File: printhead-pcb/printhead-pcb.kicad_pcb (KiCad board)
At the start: 2 copper layers, 35 x 35 mm, 4 parts, among them U3 EMC2302-2-AIZL-TR, U4 EMC2302-2-AIZL-TR, U5 ADS1015IDGS, U6 PCA9536D

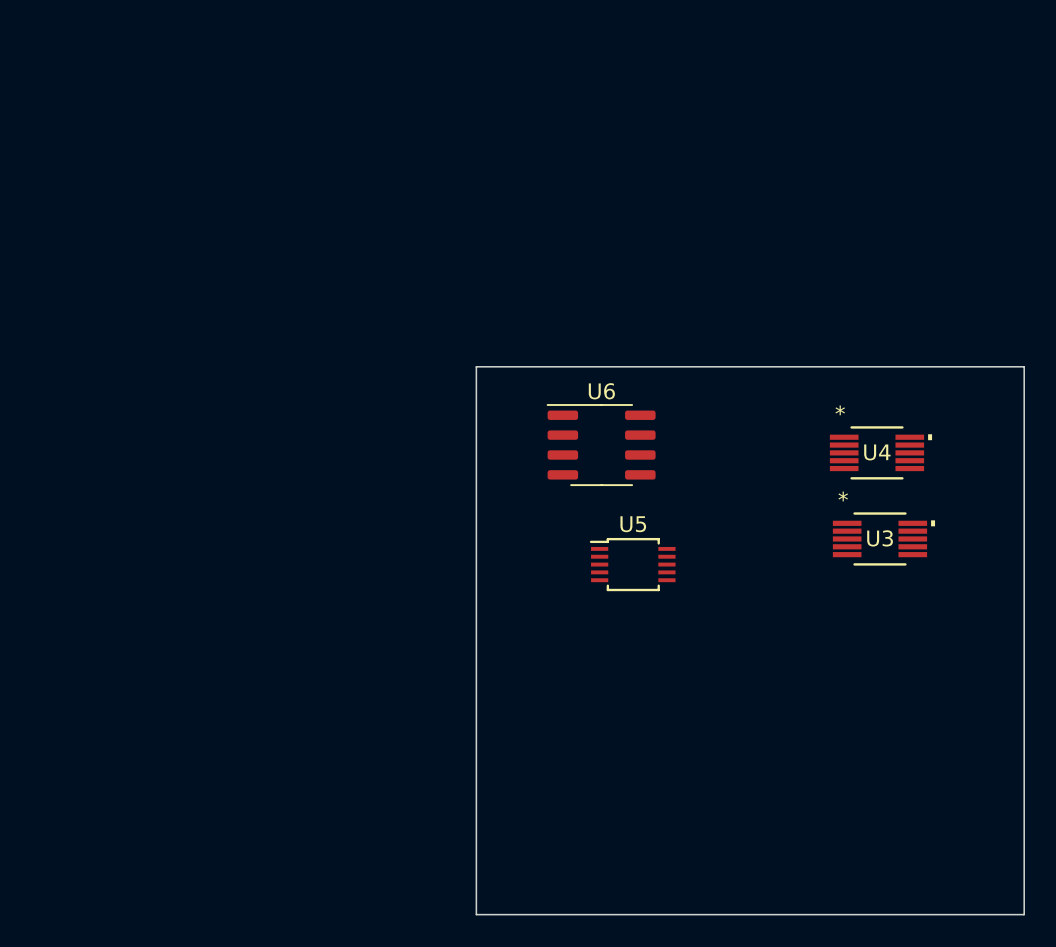
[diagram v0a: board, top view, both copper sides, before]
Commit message: circuit finished?
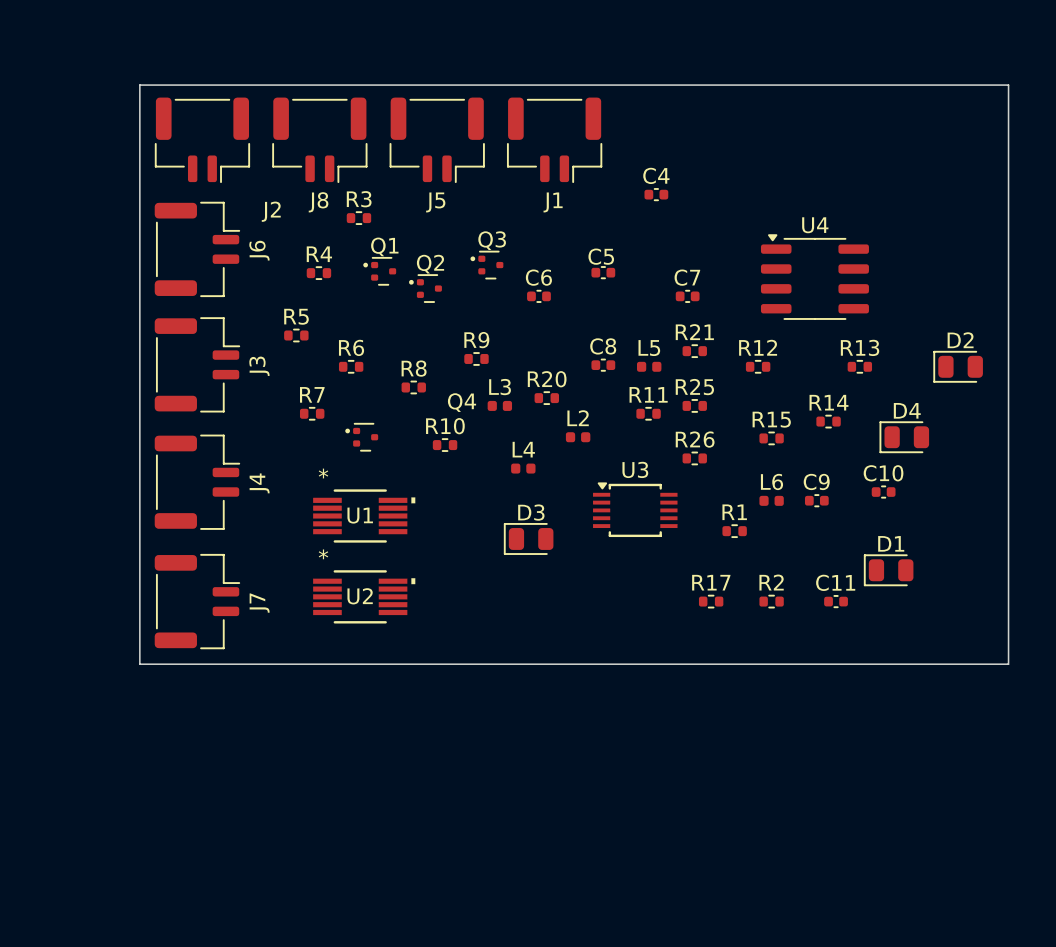
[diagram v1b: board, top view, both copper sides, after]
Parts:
- removed U5: ADS1015IDGS, Package_SO:TSSOP-10_3x3mm_P0.5mm
- removed U6: PCA9536D, Package_SO:SOIC-8_3.9x4.9mm_P1.27mm
- added C10: 0.22µF, Capacitor_SMD:C_0402_1005Metric, F.Cu at (154.0, 74.5)
- added C11: 0.1µF, Capacitor_SMD:C_0402_1005Metric, F.Cu at (151.0, 81.5)
- added C4: 0.1µF, Capacitor_SMD:C_0402_1005Metric, F.Cu at (139.5, 55.5)
- added C5: 0.1µF, Capacitor_SMD:C_0402_1005Metric, F.Cu at (136.1, 60.5)
- added C6: 0.1µF, Capacitor_SMD:C_0402_1005Metric, F.Cu at (132.0, 62.0)
- added C7: 0.1µFC, Capacitor_SMD:C_0402_1005Metric, F.Cu at (141.5, 62.0)
- added C8: 0.1µF, Capacitor_SMD:C_0402_1005Metric, F.Cu at (136.1, 66.4)
- added C9: 1µF, Capacitor_SMD:C_0402_1005Metric, F.Cu at (149.8, 75.1)
- added D1: GREEN, LED_SMD:LED_0805_2012Metric, F.Cu at (154.5, 79.5)
- added D2: YELLOW, LED_SMD:LED_0805_2012Metric, F.Cu at (158.9, 66.5)
- added D3: BLUE, LED_SMD:LED_0805_2012Metric, F.Cu at (131.5, 77.5)
- added D4: YELLOW, LED_SMD:LED_0805_2012Metric, F.Cu at (155.5, 71.0)
- added J1: FAN0, Connector_JST:JST_GH_SM02B-GHS-TB_1x02-1MP_P1.25mm_Horizontal, F.Cu at (133.0, 52.0)
- added J2: FAN2, Connector_JST:JST_GH_SM02B-GHS-TB_1x02-1MP_P1.25mm_Horizontal, F.Cu at (110.5, 52.0)
- added J3: FAN1, Connector_JST:JST_GH_SM02B-GHS-TB_1x02-1MP_P1.25mm_Horizontal, F.Cu at (110.2, 66.4)
- added J4: FAN3, Connector_JST:JST_GH_SM02B-GHS-TB_1x02-1MP_P1.25mm_Horizontal, F.Cu at (110.2, 73.9)
- added J5: T0, Connector_JST:JST_GH_SM02B-GHS-TB_1x02-1MP_P1.25mm_Horizontal, F.Cu at (125.5, 52.0)
- added J6: T1, Connector_JST:JST_GH_SM02B-GHS-TB_1x02-1MP_P1.25mm_Horizontal, F.Cu at (110.2, 59.0)
- added J7: T2, Connector_JST:JST_GH_SM02B-GHS-TB_1x02-1MP_P1.25mm_Horizontal, F.Cu at (110.2, 81.5)
- added J8: T3, Connector_JST:JST_GH_SM02B-GHS-TB_1x02-1MP_P1.25mm_Horizontal, F.Cu at (118.0, 52.0)
- added L2: L, Inductor_SMD:L_0402_1005Metric, F.Cu at (134.5, 71.0)
- added L3: L, Inductor_SMD:L_0402_1005Metric, F.Cu at (129.5, 69.0)
- added L4: L, Inductor_SMD:L_0402_1005Metric, F.Cu at (131.0, 73.0)
- added L5: L, Inductor_SMD:L_0402_1005Metric, F.Cu at (139.0, 66.5)
- added L6: L, Inductor_SMD:L_0402_1005Metric, F.Cu at (146.9, 75.1)
- added Q1: DTC143E, Package_TO_SOT_SMD:SOT-723, F.Cu at (122.1, 60.4)
- added Q2: DTC143E, Package_TO_SOT_SMD:SOT-723, F.Cu at (125.0, 61.5)
- added Q3: DTC143E, Package_TO_SOT_SMD:SOT-723, F.Cu at (128.9, 60.0)
- added Q4: DTC143E, Package_TO_SOT_SMD:SOT-723, F.Cu at (120.9, 71.0)
- added R1: 10k, Resistor_SMD:R_0402_1005Metric, F.Cu at (144.5, 77.0)
- added R10: 10k, Resistor_SMD:R_0402_1005Metric, F.Cu at (126.0, 71.5)
- added R11: 330, Resistor_SMD:R_0402_1005Metric, F.Cu at (139.0, 69.5)
- added R12: 330, Resistor_SMD:R_0402_1005Metric, F.Cu at (146.0, 66.5)
- added R13: 330, Resistor_SMD:R_0402_1005Metric, F.Cu at (152.5, 66.5)
- added R14: 10k, Resistor_SMD:R_0402_1005Metric, F.Cu at (150.5, 70.0)
- added R15: 10k, Resistor_SMD:R_0402_1005Metric, F.Cu at (146.9, 71.1)
- added R17: 1k, Resistor_SMD:R_0402_1005Metric, F.Cu at (143.0, 81.5)
- added R2: 10k, Resistor_SMD:R_0402_1005Metric, F.Cu at (146.9, 81.5)
- added R20: 1k8, Resistor_SMD:R_0402_1005Metric, F.Cu at (132.5, 68.5)
- added R21: 1k8, Resistor_SMD:R_0402_1005Metric, F.Cu at (142.0, 65.5)
- added R25: 1k8, Resistor_SMD:R_0402_1005Metric, F.Cu at (142.0, 69.0)
- added R26: 1k8, Resistor_SMD:R_0402_1005Metric, F.Cu at (142.0, 72.4)
- added R3: 10k, Resistor_SMD:R_0402_1005Metric, F.Cu at (120.5, 57.0)
- added R4: 10k, Resistor_SMD:R_0402_1005Metric, F.Cu at (117.9, 60.5)
- added R5: 3k3, Resistor_SMD:R_0402_1005Metric, F.Cu at (116.5, 64.5)
- added R6: 3k3, Resistor_SMD:R_0402_1005Metric, F.Cu at (120.0, 66.5)
- added R7: 10k, Resistor_SMD:R_0402_1005Metric, F.Cu at (117.5, 69.5)
- added R8: 10k, Resistor_SMD:R_0402_1005Metric, F.Cu at (124.0, 67.8)
- added R9: 10k, Resistor_SMD:R_0402_1005Metric, F.Cu at (128.0, 66.0)
- added U1: EMC2302-1-AIZL-TR, EMC2302-1-AIZL-TR:MSOP10_MC_MCH-M, F.Cu at (120.6, 76.0)
- added U2: EMC2302-2-AIZL-TR, EMC2302-1-AIZL-TR:MSOP10_MC_MCH-M, F.Cu at (120.6, 81.2)
- U3: value EMC2302-2-AIZL-TR -> ADS1015IDGS; footprint EMC2302-2-AIZL-TR:MSOP10_MC_MCH-M -> Package_SO:TSSOP-10_3x3mm_P0.5mm
- U4: value EMC2302-2-AIZL-TR -> PCA9536D; footprint EMC2302-2-AIZL-TR:MSOP10_MC_MCH-M -> Package_SO:SOIC-8_3.9x4.9mm_P1.27mm
- moved U3 15.7 mm to (138.2, 75.7)
- moved U4 11.8 mm to (149.6, 60.9)
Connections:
- U3 pad 1: unconnected-(U3-SMDATA-Pad1) -> GND
- U3 pad 10: unconnected-(U3-*ALERT-Pad10) -> SCL
- U3 pad 2: unconnected-(U3-SMCLK-Pad2) -> Net-(D3-A)
- U3 pad 3: unconnected-(U3-VDD-Pad3) -> GND
- U3 pad 4: unconnected-(U3-GND-Pad4) -> ADC0
- U3 pad 5: unconnected-(U3-PWM1-Pad5) -> ADC1
- U3 pad 6: unconnected-(U3-TACH1-Pad6) -> ADC2
- U3 pad 7: unconnected-(U3-PWM2-Pad7) -> ADC3
- U3 pad 8: unconnected-(U3-TACH2-Pad8) -> +3.3V
- U3 pad 9: unconnected-(U3-CLK-Pad9) -> SDA
- U4 pad 1: unconnected-(U4-SMDATA-Pad1) -> IO0
- U4 pad 2: unconnected-(U4-SMCLK-Pad2) -> IO1
- U4 pad 3: unconnected-(U4-VDD-Pad3) -> IO2
- U4 pad 4: unconnected-(U4-GND-Pad4) -> GND
- U4 pad 5: unconnected-(U4-PWM1-Pad5) -> IO3
- U4 pad 6: unconnected-(U4-TACH1-Pad6) -> SDA
- U4 pad 7: unconnected-(U4-PWM2-Pad7) -> SDA
- U4 pad 8: unconnected-(U4-TACH2-Pad8) -> +3.3V
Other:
- board size 35 x 35 mm -> 55.5 x 37 mm
- board text added: "*"

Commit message: layout
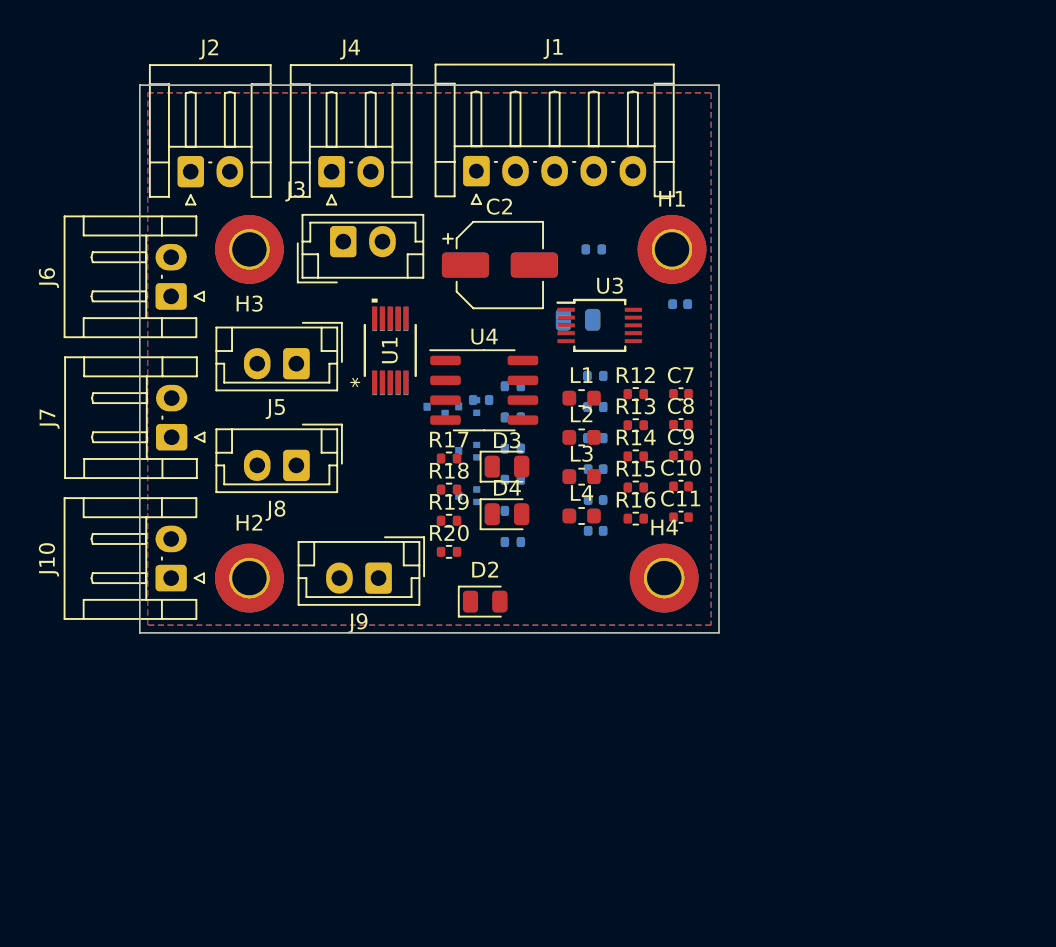
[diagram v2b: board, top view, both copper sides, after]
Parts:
- removed L5, L6: L, Inductor_SMD:L_0402_1005Metric
- removed R21, R25, R26: 1k8, Resistor_SMD:R_0402_1005Metric
- added C1: 0.1µF, Capacitor_SMD:CP_Elec_5x3, B.Cu at (129.5, 60.0)
- added C2: 0.1µF, Capacitor_SMD:CP_Elec_5x3, F.Cu at (129.5, 60.0)
- added C3: 0.22µF, Capacitor_SMD:C_0402_1005Metric, B.Cu at (135.6, 75.0)
- added H1: MountingHole_Pad, MountingHole:MountingHole_2.2mm_M2_Pad_TopBottom, F.Cu at (140.5, 59.0)
- added H2: MountingHole_Pad, MountingHole:MountingHole_2.2mm_M2_Pad_TopBottom, F.Cu at (113.5, 80.0)
- added H3: MountingHole_Pad, MountingHole:MountingHole_2.2mm_M2_Pad_TopBottom, F.Cu at (113.5, 59.0)
- added H4: MountingHole_Pad, MountingHole:MountingHole_2.2mm_M2_Pad_TopBottom, F.Cu at (140.0, 80.0)
- added J1: PWR, Connector_JST:JST_EH_S5B-EH_1x05_P2.50mm_Horizontal, F.Cu at (128.0, 54.0)
- added J10: BL_TOUCH, Connector_JST:JST_EH_S2B-EH_1x02_P2.50mm_Horizontal, F.Cu at (108.5, 80.0)
- added L1: L, Inductor_SMD:L_0603_1608Metric, F.Cu at (134.7, 68.5)
- added R16: 4k7, Resistor_SMD:R_0402_1005Metric, F.Cu at (138.2, 76.2)
- added R18: 10k, Resistor_SMD:R_0402_1005Metric, F.Cu at (126.3, 74.3)
- added R19: 330, Resistor_SMD:R_0402_1005Metric, F.Cu at (126.3, 76.3)
- C10: value 0.22µF -> 0.1µFC
- C4: value 0.1µF -> 0.22µF; moved to B.Cu
- C5, C6, D1, Q1, Q2, Q3, Q4, R10, R2, R3, R4, R7, R8, R9: moved to B.Cu
- C7: value 0.1µFC -> 0.1µF
- C9: value 1µF -> 0.1µF
- D2: value YELLOW -> BLUE
- D3: value BLUE -> YELLOW
- J2: renamed from J1; footprint Connector_JST:JST_GH_SM02B-GHS-TB_1x02-1MP_P1.25mm_Horizontal -> Connector_JST:JST_EH_S2B-EH_1x02_P2.50mm_Horizontal
- J3: renamed from J2; footprint Connector_JST:JST_GH_SM02B-GHS-TB_1x02-1MP_P1.25mm_Horizontal -> Connector_JST:JST_EH_B2B-EH-A_1x02_P2.50mm_Vertical
- J4: renamed from J3; footprint Connector_JST:JST_GH_SM02B-GHS-TB_1x02-1MP_P1.25mm_Horizontal -> Connector_JST:JST_EH_S2B-EH_1x02_P2.50mm_Horizontal
- J5: renamed from J4; footprint Connector_JST:JST_GH_SM02B-GHS-TB_1x02-1MP_P1.25mm_Horizontal -> Connector_JST:JST_EH_B2B-EH-A_1x02_P2.50mm_Vertical
- J6: renamed from J5; footprint Connector_JST:JST_GH_SM02B-GHS-TB_1x02-1MP_P1.25mm_Horizontal -> Connector_JST:JST_EH_S2B-EH_1x02_P2.50mm_Horizontal
- J7: renamed from J6; footprint Connector_JST:JST_GH_SM02B-GHS-TB_1x02-1MP_P1.25mm_Horizontal -> Connector_JST:JST_EH_S2B-EH_1x02_P2.50mm_Horizontal
- J8: renamed from J7; footprint Connector_JST:JST_GH_SM02B-GHS-TB_1x02-1MP_P1.25mm_Horizontal -> Connector_JST:JST_EH_B2B-EH-A_1x02_P2.50mm_Vertical
- J9: renamed from J8; footprint Connector_JST:JST_GH_SM02B-GHS-TB_1x02-1MP_P1.25mm_Horizontal -> Connector_JST:JST_EH_B2B-EH-A_1x02_P2.50mm_Vertical
- L2, L3, L4: footprint Inductor_SMD:L_0402_1005Metric -> Inductor_SMD:L_0603_1608Metric
- R1: value 10k -> 1k; moved to B.Cu
- R11: value 330 -> 10k; moved to B.Cu
- R12, R13: value 330 -> 4k7
- R14: value 10k -> 330
- R15: value 10k -> 4k7
- R17: value 1k -> 10k
- R20: value 1k8 -> 330
- R5, R6: value 3k3 -> 10k; moved to B.Cu
- U1: value EMC2302-1-AIZL-TR -> EMC2302-2-AIZL-TR; footprint EMC2302-1-AIZL-TR:MSOP10_MC_MCH-M -> EMC2302-2-AIZL-TR:MSOP10_MC_MCH
- U2: footprint EMC2302-1-AIZL-TR:MSOP10_MC_MCH-M -> EMC2302-2-AIZL-TR:MSOP10_MC_MCH; moved to B.Cu
- moved D2 33.9 mm to (128.6, 81.5)
- moved J9 28.2 mm to (121.8, 80.0)
- moved D4 26.0 mm to (130.0, 75.9)
- moved D1 25.6 mm to (134.5, 63.5), turned to 180 degrees
- moved J2 23.3 mm to (109.8, 54.0), turned to 0 degrees
- moved U4 22.3 mm to (128.5, 68.0)
- moved R3 20.6 mm to (135.6, 71.1), turned to 180 degrees
- moved J6 19.7 mm to (108.5, 62.0), turned to 90 degrees
- moved R17 19.1 mm to (126.3, 72.4)
- moved C4 18.0 mm to (135.6, 73.0), turned to 180 degrees
- moved R2 16.8 mm to (135.6, 69.1), turned to 180 degrees
- moved U2 15.8 mm to (122.5, 65.5), turned to -90 degrees
- moved C6 15.4 mm to (135.6, 77.0), turned to 180 degrees
- moved J4 15.0 mm to (118.8, 54.0), turned to 0 degrees
- moved R13 14.8 mm to (138.2, 70.2)
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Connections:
- C10 pad 1: Net-(C10-Pad1) -> ADC2
- C11 pad 1: Net-(C10-Pad1) -> ADC3
- C4 pad 1: ADC0 -> +3V3
- C5 pad 1: +3.3V -> +12V
- C6 pad 1: ADC0 -> +3V3
- C8 pad 1: ADC0 -> +3.3V
- C9 pad 1: Net-(C10-Pad1) -> ADC1
- D2 pad 2: IO0 -> Net-(D2-A)
- D3 pad 2: Net-(D3-A) -> IO0
- L2 pad 1: TC0 -> TC1
- L2 pad 2: ADC0 -> ADC1
- L3 pad 1: TC0 -> TC2
- L3 pad 2: ADC0 -> ADC2
- L4 pad 1: TC0 -> TC3
- L4 pad 2: ADC0 -> ADC3
- R1 pad 1: +3V3 -> Net-(D1-K)
- R1 pad 2: SDA -> GND
- R10 pad 1: Net-(U2-CLK) -> Net-(U1-CLK)
- R11 pad 1: GND -> Net-(U2-CLK)
- R11 pad 2: Net-(D3-K) -> GND
- R12 pad 1: Net-(D2-K) -> AREF
- R12 pad 2: GND -> ADC0
- R13 pad 1: Net-(D4-K) -> AREF
- R13 pad 2: GND -> ADC1
- R14 pad 1: IO2 -> GND
- R14 pad 2: GND -> Net-(D2-K)
- R15 pad 1: IO3 -> AREF
- R15 pad 2: GND -> ADC2
- R17 pad 1: Net-(D1-K) -> IO3
- R2 pad 2: SCL -> SDA
- R20 pad 1: AREF -> Net-(D4-K)
- R20 pad 2: ADC0 -> GND
- R3 pad 1: Net-(U1-TACH1) -> +3V3
- R3 pad 2: GND -> SCL
- R4 pad 1: Net-(U2-TACH1) -> Net-(U1-TACH1)
- R5 pad 1: Net-(U1-*ALERT) -> Net-(U2-TACH1)
- R6 pad 1: Net-(U2-*ALERT) -> Net-(U1-*ALERT)
- R7 pad 1: Net-(U1-TACH2) -> Net-(U2-*ALERT)
- R8 pad 1: Net-(U2-TACH2) -> Net-(U1-TACH2)
- R9 pad 1: Net-(U1-CLK) -> Net-(U2-TACH2)
- U3 pad 2: Net-(D3-A) -> Net-(D2-A)
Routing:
- added copper zone on B.Cu, net GND
- added copper zone on F.Cu, net GND
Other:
- board size 55.5 x 37 mm -> 37 x 35 mm
- board text removed: "*"

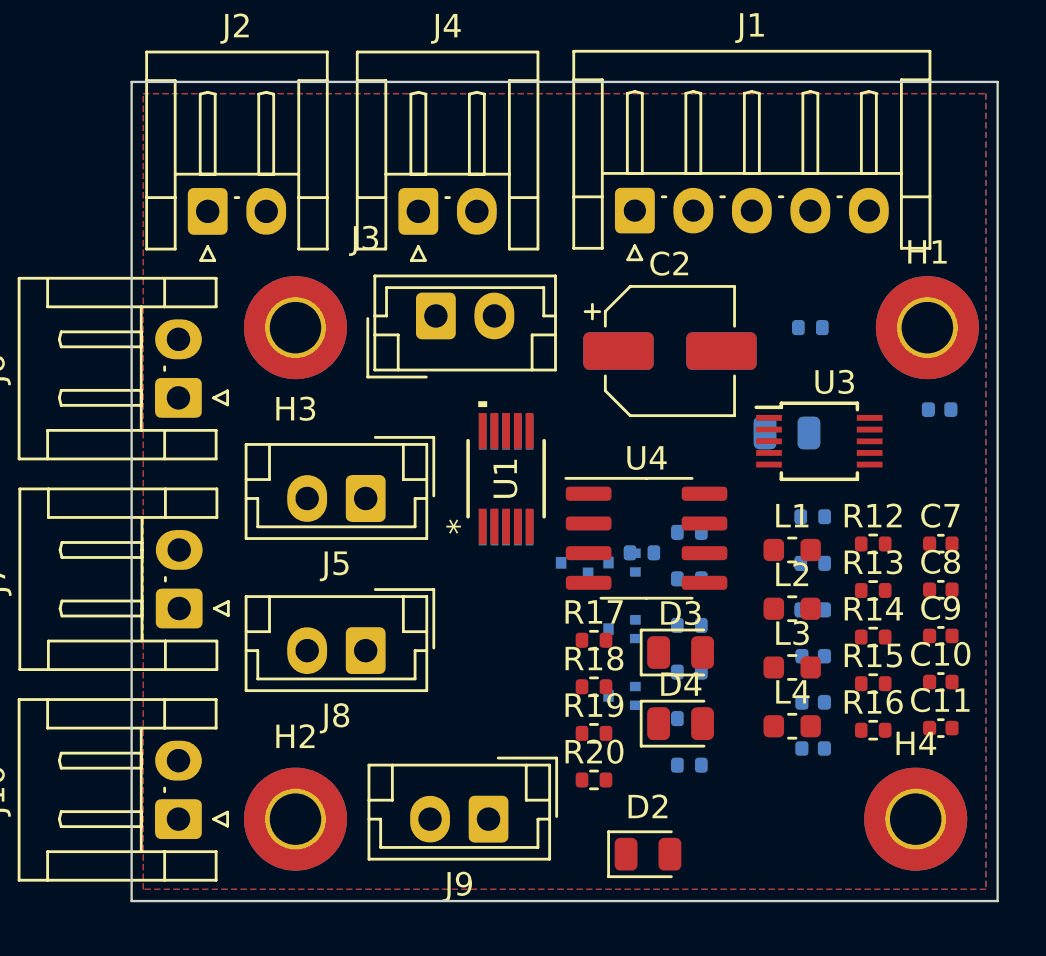
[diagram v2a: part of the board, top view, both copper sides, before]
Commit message: first pcb layout
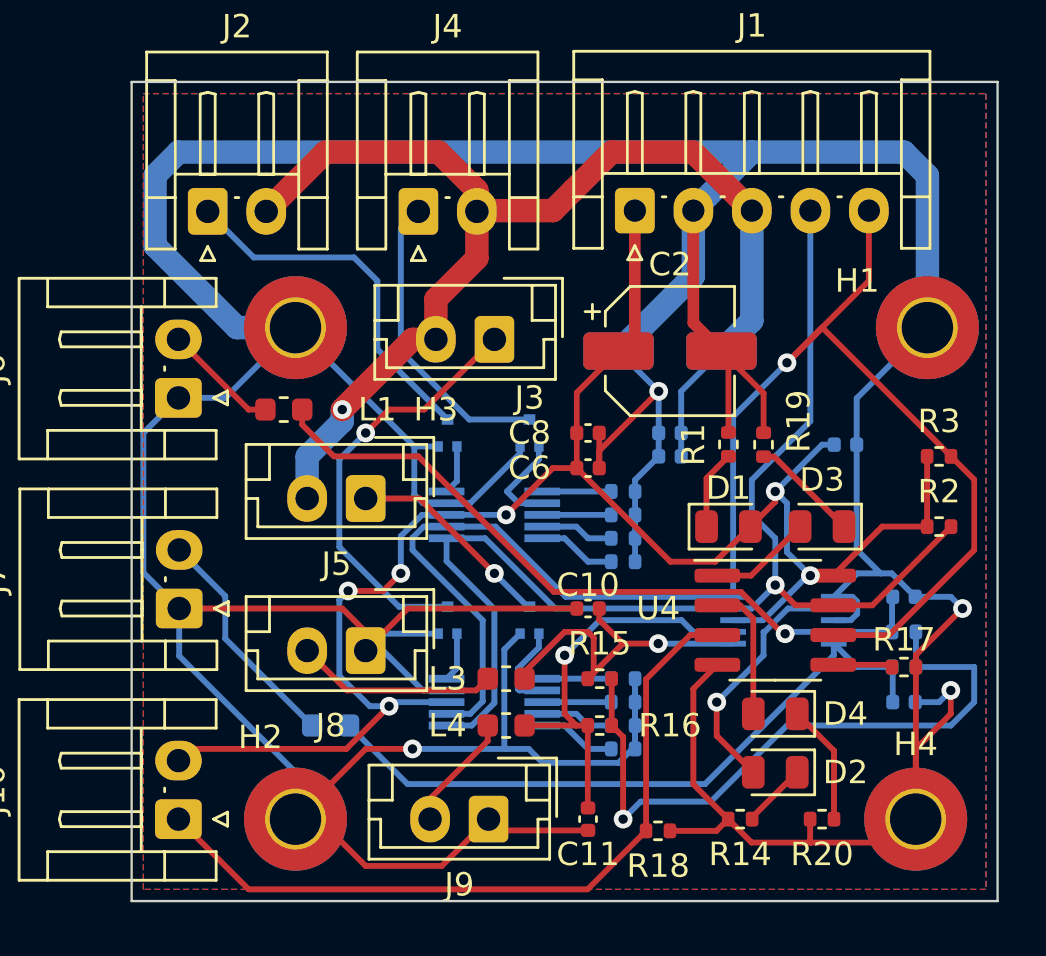
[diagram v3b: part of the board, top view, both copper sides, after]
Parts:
- C6, D1, R1, R2, R3: moved to F.Cu
- C7, C9, L2, R12, R13, U1, U3: moved to B.Cu
- moved L1 22.5 mm to (113.0, 62.5)
- moved L2 20.3 mm to (115.0, 76.0)
- moved R11 18.8 mm to (127.5, 76.0), turned to 0 degrees
- moved C8 16.5 mm to (126.0, 63.5)
- moved C11 15.6 mm to (126.0, 80.0), turned to -90 degrees
- moved C10 15.4 mm to (126.0, 71.0), turned to 180 degrees
- moved C6 15.4 mm to (126.0, 65.0), turned to 0 degrees
- moved R19 14.3 mm to (133.5, 64.0), turned to 90 degrees
- moved R17 13.3 mm to (139.5, 73.5)
- moved C3 13.0 mm to (129.5, 63.5)
- moved L3 12.2 mm to (122.5, 74.0)
- moved L4 12.2 mm to (122.5, 76.0)
- moved C5 11.7 mm to (129.5, 64.5)
- moved R15 11.7 mm to (126.5, 74.0), turned to 180 degrees
- moved R16 11.7 mm to (126.5, 76.0), turned to 180 degrees
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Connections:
- C8 pad 1: +3.3V -> +3V3
- J10 pad 1: GND -> IO2
- J10 pad 2: IO2 -> +3V3
- U3 pad 8: +3.3V -> +3V3
- U4 pad 6: SDA -> SCL
- U4 pad 8: +3.3V -> +3V3
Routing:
- net GND: track 0.00 -> 265.1 mm, vias 0 -> 4
- net +3V3: track 0.00 -> 76.0 mm, vias 0 -> 6
- net SCL: track 0.00 -> 65.9 mm, vias 0 -> 1
- net +12V: track 0.00 -> 53.1 mm, vias 0 -> 1
- net SDA: track 0.00 -> 52.7 mm, vias 0 -> 1
- net IO2: track 0.00 -> 32.6 mm
- net ADC0: track 0.00 -> 31.1 mm, vias 0 -> 1
- net ADC1: track 0.00 -> 28.9 mm
- net AREF: track 0.00 -> 28.8 mm, vias 0 -> 1
- net Net-(J3-Pin_1): track 0.00 -> 18.2 mm, vias 0 -> 1
- net ADC3: track 0.00 -> 17.5 mm, vias 0 -> 1
- net Net-(J2-Pin_1): track 0.00 -> 15.6 mm
- net ADC2: track 0.00 -> 14.7 mm, vias 0 -> 1
- net Net-(J4-Pin_1): track 0.00 -> 13.0 mm
- net Net-(D2-A): track 0.00 -> 10.9 mm, vias 0 -> 1
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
